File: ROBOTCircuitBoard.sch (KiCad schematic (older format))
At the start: 32 parts, among them J1 DB15_HighDensity_MountingHoles, J2 DB15_HighDensity_MountingHoles, P1 CONN_01X03, P2 CONN_01X04, P5 CONN_01X05, U1 MCP2551-I/P

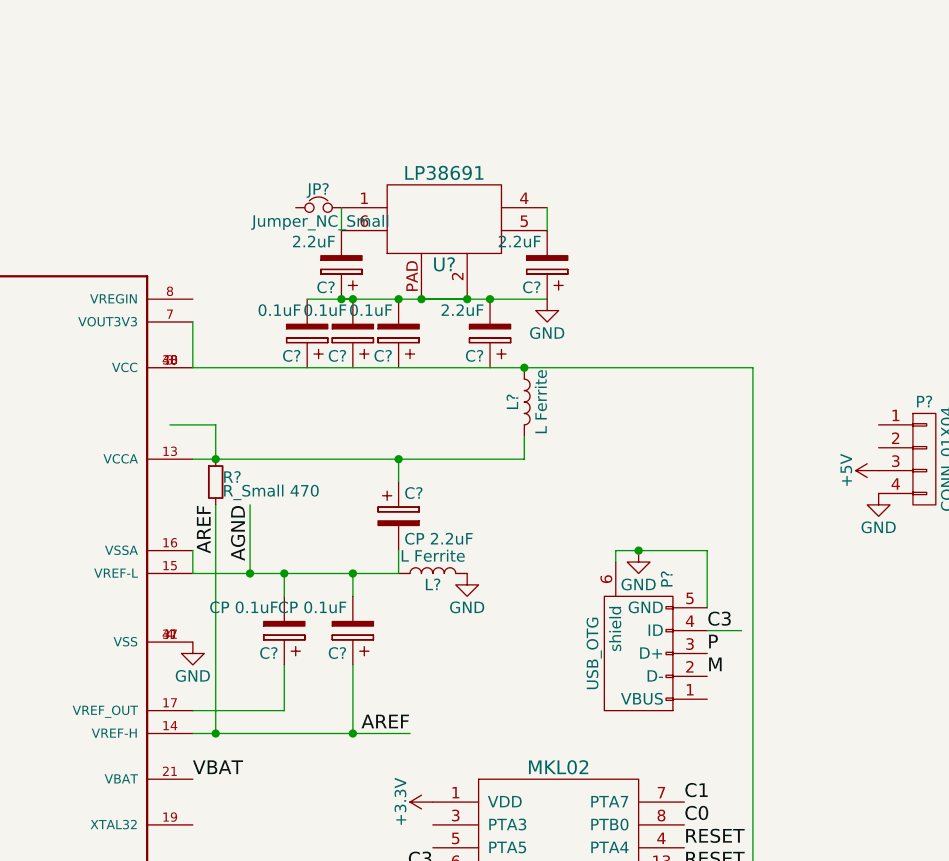
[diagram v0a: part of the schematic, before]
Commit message: finished schematic draft 1
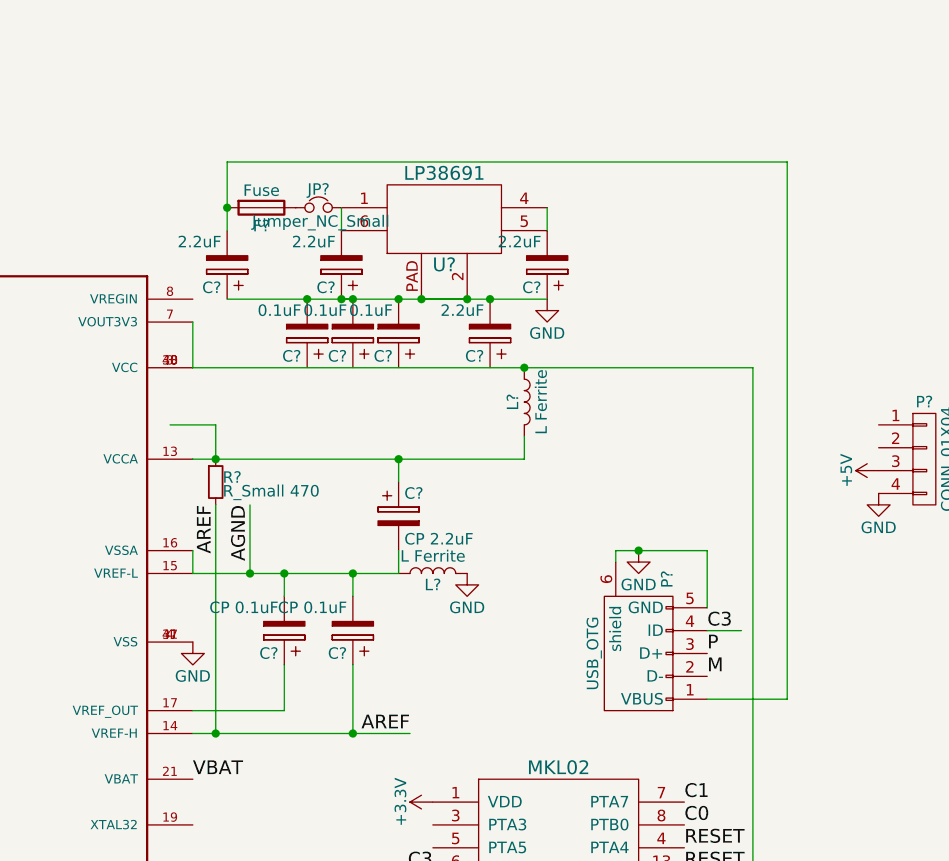
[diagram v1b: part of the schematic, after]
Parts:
- added C?: 2.2uF, symbol CP
- added F?: Fuse, symbol Fuse
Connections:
- wire segments 86 -> 90
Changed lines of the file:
@@
 	4700 6350 4700 6450
 Wire Wire Line
-	4150 3450 5200 3450
+	3800 3450 5200 3450
 Connection ~ 4950 3450
 Connection ~ 4550 3450
@@
 	1    0    0    -1
 $EndComp
+$Comp
+L Fuse F?
+U 1 1 5980A7D8
+P 3950 3050
+F 0 "F?" V 4030 3050 50  0000 C CNN
+F 1 "Fuse" V 3875 3050 50  0000 C CNN
+F 2 "" V 3880 3050 50  0000 C CNN
+F 3 "" H 3950 3050 50  0000 C CNN
+	1    3950 3050
+	0    1    1    0
+$EndComp
+Connection ~ 4150 3450
+$Comp
+L CP C?
+U 1 1 5980AC81
+P 3800 3300
+F 0 "C?" H 3825 3400 50  0000 L CNN
+F 1 "2.2uF" H 3825 3200 50  0000 L CNN
+F 2 "" H 3838 3150 50  0000 C CNN
+F 3 "" H 3800 3300 50  0000 C CNN
+	1    3800 3300
+	-1   0    0    1
+$EndComp
+Wire Wire Line
+	3800 2850 3800 3150
+Wire Wire Line
+	3800 2850 6250 2850
+Wire Wire Line
+	6250 2850 6250 5200
+Wire Wire Line
+	6250 5200 5900 5200
+Connection ~ 3800 3050
 $EndSCHEMATC
